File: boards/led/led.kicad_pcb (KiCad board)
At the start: 2 copper layers, 72.4 x 27.9 mm, 5 parts, among them J1 RJ45, P1 CONN_01X08

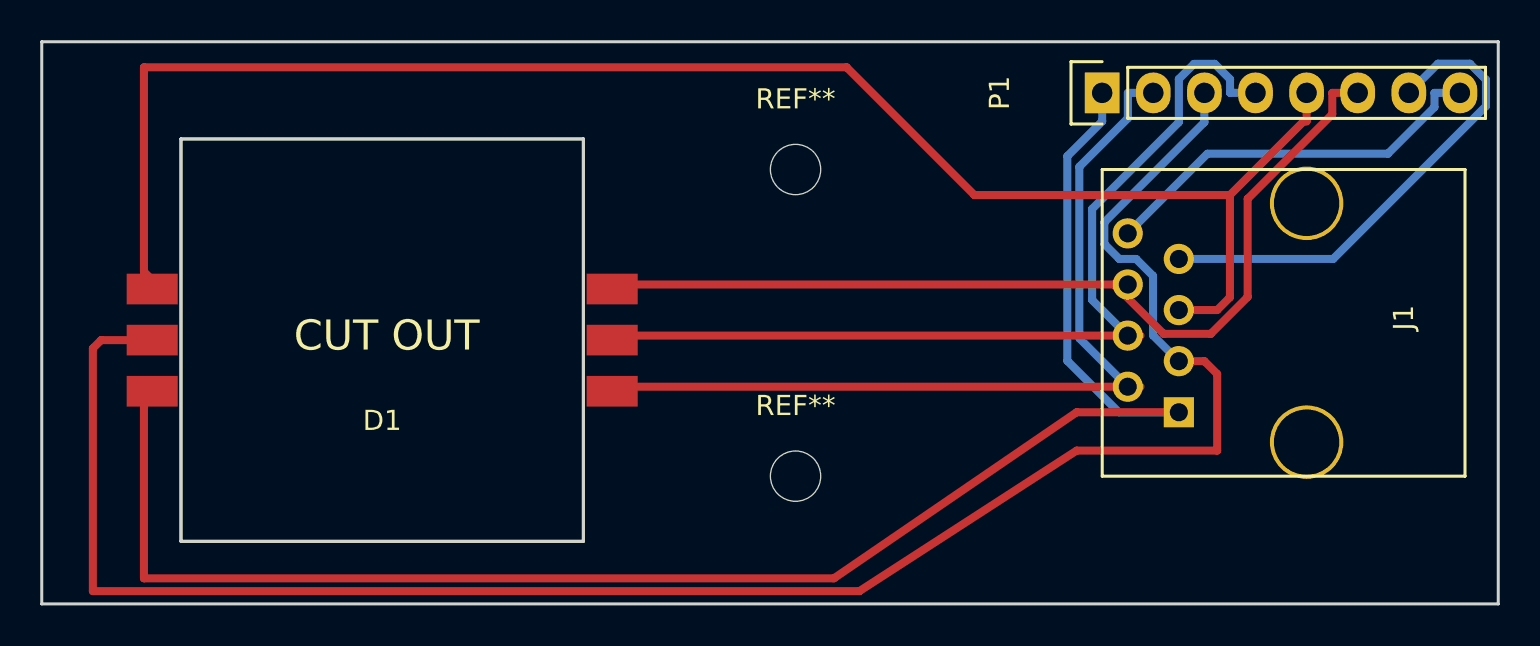
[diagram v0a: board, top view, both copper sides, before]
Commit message: final changes
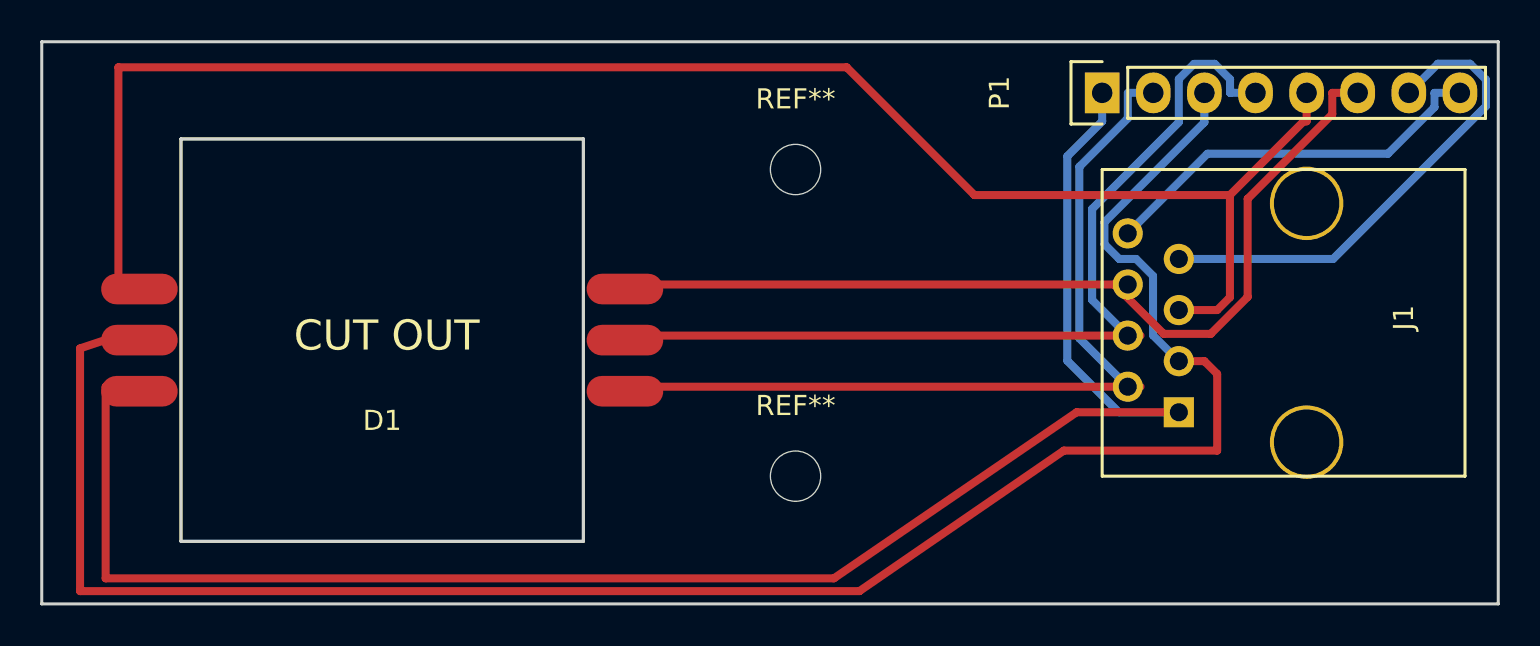
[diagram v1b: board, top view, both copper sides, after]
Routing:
- net Net-(D1-Pad1): track 84.1 -> 88.4 mm
- net Net-(D1-Pad3): track 82.4 -> 85.4 mm
- net Net-(D1-Pad2): track 96.5 -> 97.8 mm
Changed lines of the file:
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@@
     (pad 1 thru_hole circle (at 0 0) (size 2.5 2.5) (drill 2.5) (layers))
-  )
-  (module lighting:10wled (layer F.Cu)
-    (at 149 105)
-    (fp_text reference D1 (at 0 4) (layer F.SilkS)
-      (effects (font (size 1 1) (thickness 0.15)))
-    )
-    (fp_text value LED_RGB (at 0 -4) (layer F.Fab)
-      (effects (font (size 1 1) (thickness 0.15)))
-    )
-    (fp_line (start -10 -10) (end 10 -10) (layer F.SilkS) (width 0.15))
-    (fp_line (start 10 -10) (end 10 10) (layer F.SilkS) (width 0.15))
-    (fp_line (start 10 10) (end -10 10) (layer F.SilkS) (width 0.15))
-    (fp_line (start -10 10) (end -10 -10) (layer F.SilkS) (width 0.15))
-    (pad 2 smd rect (at -11.43 0) (size 2.54 1.524) (layers F.Cu F.Paste F.Mask)
-      (net 1 "Net-(D1-Pad2)"))
-    (pad 3 smd rect (at -11.43 -2.54) (size 2.54 1.524) (layers F.Cu F.Paste F.Mask)
-      (net 2 "Net-(D1-Pad3)"))
-    (pad 1 smd rect (at -11.43 2.54) (size 2.54 1.524) (layers F.Cu F.Paste F.Mask)
-      (net 3 "Net-(D1-Pad1)"))
-    (pad 6 smd rect (at 11.43 2.54) (size 2.54 1.524) (layers F.Cu F.Paste F.Mask)
-      (net 4 "Net-(D1-Pad6)"))
-    (pad 5 smd rect (at 11.43 0) (size 2.54 1.524) (layers F.Cu F.Paste F.Mask)
-      (net 5 "Net-(D1-Pad5)"))
-    (pad 4 smd rect (at 11.43 -2.54) (size 2.54 1.524) (layers F.Cu F.Paste F.Mask)
-      (net 6 "Net-(D1-Pad4)"))
   )
   (module Pin_Headers:Pin_Header_Straight_1x08 (layer F.Cu)
@@
     (pad 1 thru_hole circle (at 0 0) (size 2.5 2.5) (drill 2.5) (layers))
   )
+  (module lighting:10wled (layer F.Cu)
+    (at 149 105)
+    (fp_text reference D1 (at 0 4) (layer F.SilkS)
+      (effects (font (size 1 1) (thickness 0.15)))
+    )
+    (fp_text value LED_RGB (at 0 -4) (layer F.Fab)
+      (effects (font (size 1 1) (thickness 0.15)))
+    )
+    (fp_line (start -10 -10) (end 10 -10) (layer F.SilkS) (width 0.15))
+    (fp_line (start 10 -10) (end 10 10) (layer F.SilkS) (width 0.15))
+    (fp_line (start 10 10) (end -10 10) (layer F.SilkS) (width 0.15))
+    (fp_line (start -10 10) (end -10 -10) (layer F.SilkS) (width 0.15))
+    (pad 2 smd oval (at -12.065 0) (size 3.81 1.524) (layers F.Cu F.Paste F.Mask)
+      (net 1 "Net-(D1-Pad2)"))
+    (pad 3 smd oval (at -12.065 -2.54) (size 3.81 1.524) (layers F.Cu F.Paste F.Mask)
+      (net 2 "Net-(D1-Pad3)"))
+    (pad 1 smd oval (at -12.065 2.54) (size 3.81 1.524) (layers F.Cu F.Paste F.Mask)
+      (net 3 "Net-(D1-Pad1)"))
+    (pad 6 smd oval (at 12.065 2.54) (size 3.81 1.524) (layers F.Cu F.Paste F.Mask)
+      (net 4 "Net-(D1-Pad6)"))
+    (pad 5 smd oval (at 12.065 0) (size 3.81 1.524) (layers F.Cu F.Paste F.Mask)
+      (net 5 "Net-(D1-Pad5)"))
+    (pad 4 smd oval (at 12.065 -2.54) (size 3.81 1.524) (layers F.Cu F.Paste F.Mask)
+      (net 6 "Net-(D1-Pad4)"))
+  )
   (gr_line (start 132.08 118.11) (end 204.47 118.11) (angle 90) (layer Edge.Cuts) (width 0.15))
   (gr_line (start 132.08 90.17) (end 132.08 118.11) (angle 90) (layer Edge.Cuts) (width 0.15))
@@
   (segment (start 187.3123 104.7623) (end 188.595 106.045) (width 0.4) (layer B.Cu) (net 1))
   (segment (start 187.3123 101.8058) (end 187.3123 104.7623) (width 0.4) (layer B.Cu) (net 1))
-  (segment (start 135.03 105) (end 134.62 105.41) (width 0.4) (layer F.Cu) (net 1))
-  (segment (start 134.62 105.41) (end 134.62 117.475) (width 0.4) (layer F.Cu) (net 1))
-  (segment (start 134.62 117.475) (end 172.72 117.475) (width 0.4) (layer F.Cu) (net 1))
-  (segment (start 137.57 105) (end 135.03 105) (width 0.4) (layer F.Cu) (net 1))
-  (segment (start 172.72 117.475) (end 183.515 110.49) (width 0.4) (layer F.Cu) (net 1))
-  (segment (start 183.515 110.49) (end 190.5 110.49) (width 0.4) (layer F.Cu) (net 1))
+  (segment (start 135.89 104.775) (end 133.985 105.41) (width 0.4) (layer F.Cu) (net 1))
+  (segment (start 133.985 105.41) (end 133.985 117.475) (width 0.4) (layer F.Cu) (net 1))
+  (segment (start 133.985 117.475) (end 172.72 117.475) (width 0.4) (layer F.Cu) (net 1))
+  (segment (start 137.57 105) (end 135.89 104.775) (width 0.4) (layer F.Cu) (net 1))
+  (segment (start 172.72 117.475) (end 182.88 110.49) (width 0.4) (layer F.Cu) (net 1))
+  (segment (start 182.88 110.49) (end 190.5 110.49) (width 0.4) (layer F.Cu) (net 1))
   (segment (start 189.23 106.045) (end 188.595 106.045) (width 0.4) (layer F.Cu) (net 1))
   (segment (start 190.5 110.49) (end 190.5 106.68) (width 0.4) (layer F.Cu) (net 1))
@@
   (segment (start 190.5 103.505) (end 191.135 102.87) (width 0.4) (layer F.Cu) (net 2))
   (segment (start 189.23 103.505) (end 190.5 103.505) (width 0.4) (layer F.Cu) (net 2))
-  (segment (start 137.16 101.6) (end 137.57 102.01) (width 0.4) (layer F.Cu) (net 2))
-  (segment (start 137.16 91.44) (end 137.16 101.6) (width 0.4) (layer F.Cu) (net 2))
-  (segment (start 172.085 91.44) (end 137.16 91.44) (width 0.4) (layer F.Cu) (net 2))
+  (segment (start 135.89 102.235) (end 137.57 102.01) (width 0.4) (layer F.Cu) (net 2))
+  (segment (start 135.89 91.44) (end 135.89 102.235) (width 0.4) (layer F.Cu) (net 2))
+  (segment (start 172.085 91.44) (end 135.89 91.44) (width 0.4) (layer F.Cu) (net 2))
   (segment (start 178.435 97.79) (end 172.085 91.44) (width 0.4) (layer F.Cu) (net 2))
   (segment (start 191.135 97.79) (end 178.435 97.79) (width 0.4) (layer F.Cu) (net 2))
@@
   (segment (start 188.595 108.585) (end 183.515 108.585) (width 0.4) (layer F.Cu) (net 3))
   (segment (start 183.515 108.585) (end 171.45 116.84) (width 0.4) (layer F.Cu) (net 3))
-  (segment (start 171.45 116.84) (end 137.16 116.84) (width 0.4) (layer F.Cu) (net 3))
-  (segment (start 137.16 116.84) (end 137.16 107.95) (width 0.4) (layer F.Cu) (net 3))
-  (segment (start 137.16 107.95) (end 137.57 107.54) (width 0.4) (layer F.Cu) (net 3))
+  (segment (start 171.45 116.84) (end 135.255 116.84) (width 0.4) (layer F.Cu) (net 3))
+  (segment (start 135.255 116.84) (end 135.255 107.315) (width 0.4) (layer F.Cu) (net 3))
+  (segment (start 135.255 107.315) (end 137.57 107.54) (width 0.4) (layer F.Cu) (net 3))
   (segment (start 186.0611 93.9739) (end 186.0611 92.71) (width 0.4) (layer B.Cu) (net 4))
   (segment (start 183.6503 96.3847) (end 186.0611 93.9739) (width 0.4) (layer B.Cu) (net 4))

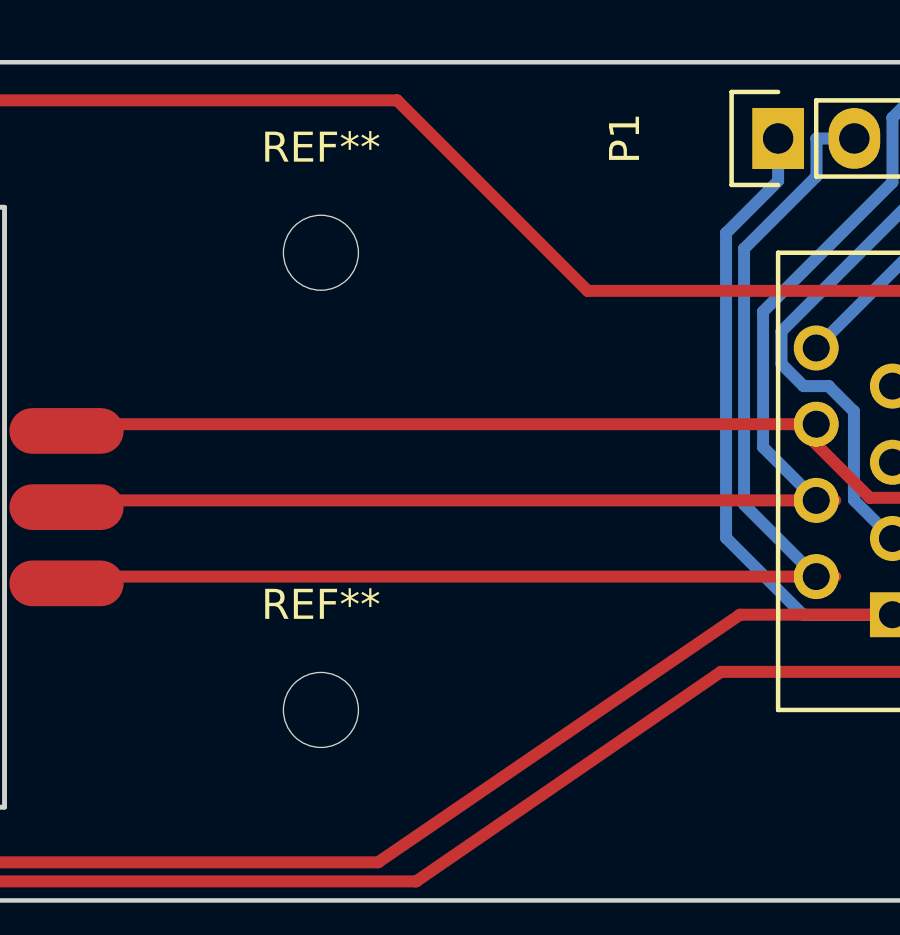
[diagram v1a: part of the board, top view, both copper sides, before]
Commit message: sink
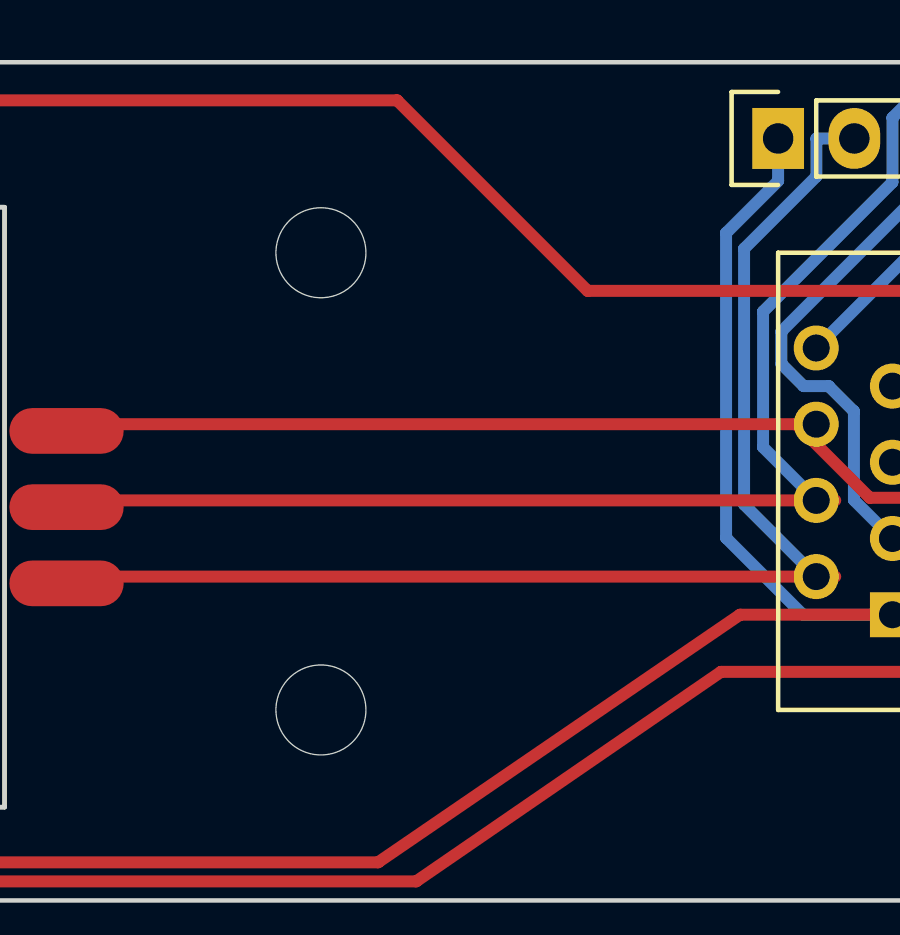
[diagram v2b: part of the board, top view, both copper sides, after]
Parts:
- REF1, REF2: renamed from REF**; footprint Mounting_Holes:MountingHole_2-5mm -> Mounting_Holes:MountingHole_3mm
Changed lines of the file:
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@@
     (links 14)
     (no_connects 0)
-    (area 132.004999 87.601666 204.560001 118.185001)
+    (area 116.420925 72.420925 204.560001 137.579075)
     (thickness 1.6)
-    (drawings 9)
+    (drawings 10)
     (tracks 84)
     (zones 0)
@@
     )
   )
-  (module Mounting_Holes:MountingHole_2-5mm (layer F.Cu)
-    (at 169.545 111.76)
-    (descr "Mounting hole, Befestigungsbohrung, 2,5mm, No Annular, Kein Restring,")
-    (tags "Mounting hole, Befestigungsbohrung, 2,5mm, No Annular, Kein Restring,")
-    (fp_text reference REF** (at 0 -3.50012) (layer F.SilkS)
-      (effects (font (size 1 1) (thickness 0.15)))
-    )
-    (fp_text value MountingHole_2-5mm (at 0.09906 3.59918) (layer F.Fab)
-      (effects (font (size 1 1) (thickness 0.15)))
-    )
-    (fp_circle (center 0 0) (end 2.5 0) (layer Cmts.User) (width 0.381))
-    (pad 1 thru_hole circle (at 0 0) (size 2.5 2.5) (drill 2.5) (layers))
-  )
   (module Pin_Headers:Pin_Header_Straight_1x08 (layer F.Cu)
     (at 184.785 92.71 90)
     (descr "Through hole pin header")
     (tags "pin header")
-    (fp_text reference P1 (at 0 -5.1 90) (layer F.SilkS)
-      (effects (font (size 1 1) (thickness 0.15)))
-    )
-    (fp_text value CONN_01X08 (at 0 -3.1 90) (layer F.Fab)
+    (fp_text reference P1 (at 0 -5.1 90) (layer F.SilkS) hide
+      (effects (font (size 1 1) (thickness 0.15)))
+    )
+    (fp_text value CONN_01X08 (at 0 -3.1 90) (layer F.Fab) hide
       (effects (font (size 1 1) (thickness 0.15)))
     )
@@
     )
   )
-  (module Mounting_Holes:MountingHole_2-5mm (layer F.Cu)
-    (at 169.545 96.52)
-    (descr "Mounting hole, Befestigungsbohrung, 2,5mm, No Annular, Kein Restring,")
-    (tags "Mounting hole, Befestigungsbohrung, 2,5mm, No Annular, Kein Restring,")
-    (fp_text reference REF** (at 0 -3.50012) (layer F.SilkS)
-      (effects (font (size 1 1) (thickness 0.15)))
-    )
-    (fp_text value MountingHole_2-5mm (at 0.09906 3.59918) (layer F.Fab)
-      (effects (font (size 1 1) (thickness 0.15)))
-    )
-    (fp_circle (center 0 0) (end 2.5 0) (layer Cmts.User) (width 0.381))
-    (pad 1 thru_hole circle (at 0 0) (size 2.5 2.5) (drill 2.5) (layers))
-  )
   (module lighting:10wled (layer F.Cu)
     (at 149 105)
@@
       (net 6 "Net-(D1-Pad4)"))
   )
+  (module Mounting_Holes:MountingHole_3mm (layer F.Cu)
+    (at 169.545 111.76)
+    (descr "Mounting hole, Befestigungsbohrung, 3mm, No Annular, Kein Restring,")
+    (tags "Mounting hole, Befestigungsbohrung, 3mm, No Annular, Kein Restring,")
+    (fp_text reference REF1 (at 0 -4.0005) (layer F.SilkS) hide
+      (effects (font (size 1 1) (thickness 0.15)))
+    )
+    (fp_text value MountingHole_2-5mm (at 1.00076 5.00126) (layer F.Fab)
+      (effects (font (size 1 1) (thickness 0.15)))
+    )
+    (fp_circle (center 0 0) (end 3 0) (layer Cmts.User) (width 0.381))
+    (pad 1 thru_hole circle (at 0 0) (size 3 3) (drill 3) (layers))
+  )
+  (module Mounting_Holes:MountingHole_3mm (layer F.Cu)
+    (at 169.545 96.52)
+    (descr "Mounting hole, Befestigungsbohrung, 3mm, No Annular, Kein Restring,")
+    (tags "Mounting hole, Befestigungsbohrung, 3mm, No Annular, Kein Restring,")
+    (fp_text reference REF2 (at 0 -4.0005) (layer F.SilkS) hide
+      (effects (font (size 1 1) (thickness 0.15)))
+    )
+    (fp_text value MountingHole_2-5mm (at 1.00076 5.00126) (layer F.Fab)
+      (effects (font (size 1 1) (thickness 0.15)))
+    )
+    (fp_circle (center 0 0) (end 3 0) (layer Cmts.User) (width 0.381))
+    (pad 1 thru_hole circle (at 0 0) (size 3 3) (drill 3) (layers))
+  )
+  (gr_circle (center 149 105) (end 177.8 120.015) (layer Dwgs.User) (width 0.2))
   (gr_line (start 132.08 118.11) (end 204.47 118.11) (angle 90) (layer Edge.Cuts) (width 0.15))
   (gr_line (start 132.08 90.17) (end 132.08 118.11) (angle 90) (layer Edge.Cuts) (width 0.15))
